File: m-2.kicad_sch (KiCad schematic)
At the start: 14 parts, among them J3 Bus_M.2_1-2199230-6, Y1 Oscillator_SMD_32.768kHz_ECS_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

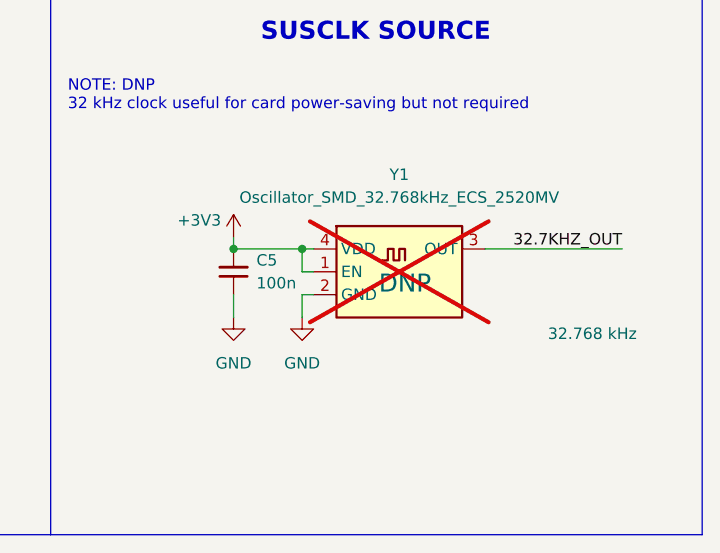
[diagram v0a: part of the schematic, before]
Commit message: [#83351] Project refresh 81589
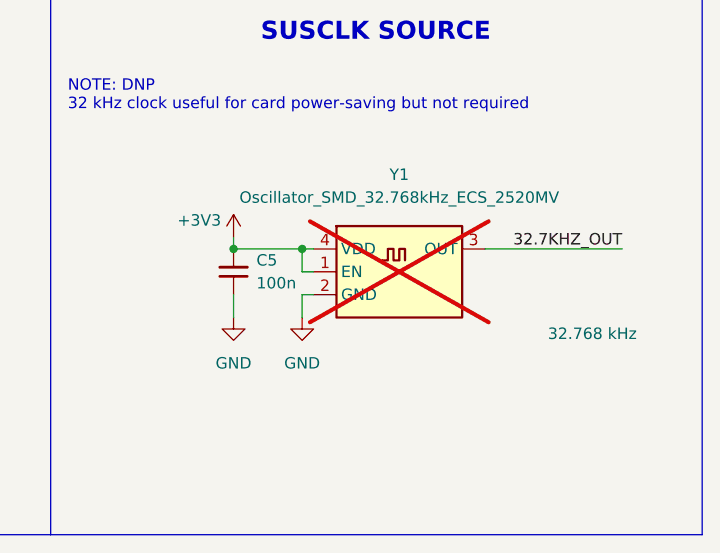
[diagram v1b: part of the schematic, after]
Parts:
- Y1: DNP DNP -> (none)
